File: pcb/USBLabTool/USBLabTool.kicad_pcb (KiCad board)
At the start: 4 copper layers, 79.4 x 56.2 mm, 236 parts, among them J1 Conn_01x06_Pin, J17 2x01, J19 T_N5V, J2 Conn_02x12_Odd_Even, J20 USB_C_Receptacle, K1 G5V-2, K2 G5V-2, Q1 STL11N3LLH6, SW1 TS02-66-73-BK-100-SCR-D, U1 AQY284SX, U10 MC33274ADR2G, U11 DG403, U12 STM32H562VGTx, U13 R1283K002A, U14 ST1L05APU33R, U15 ST1L05APU33R, U16 LTC1983ES6-5TRMPBF, U17 TCPP01-M12, U18 74HC245, U19 USBLC6-2SC6, U2 AQY284SX, U20 74HC245, U3 CD74HC4316, U4 LMP7718, U5 CD74HC4316, U6 LMP7718, U7 OPA863, U8 OPA863, U9 MC33274ADR2G, Y1 32.768kHz, Y2 NX2016SA-25M-EXS00A-CS08742

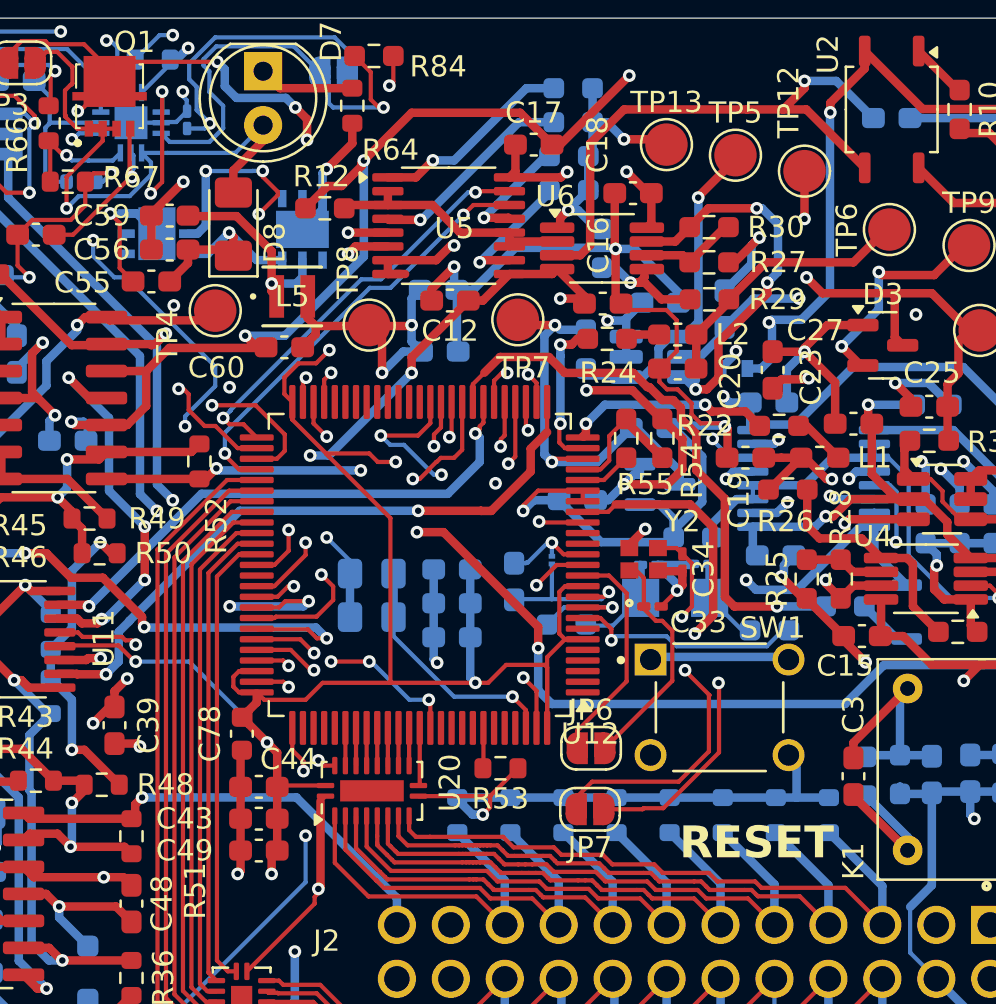
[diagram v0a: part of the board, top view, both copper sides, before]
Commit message: Update USBLabTool.kicad_pcb
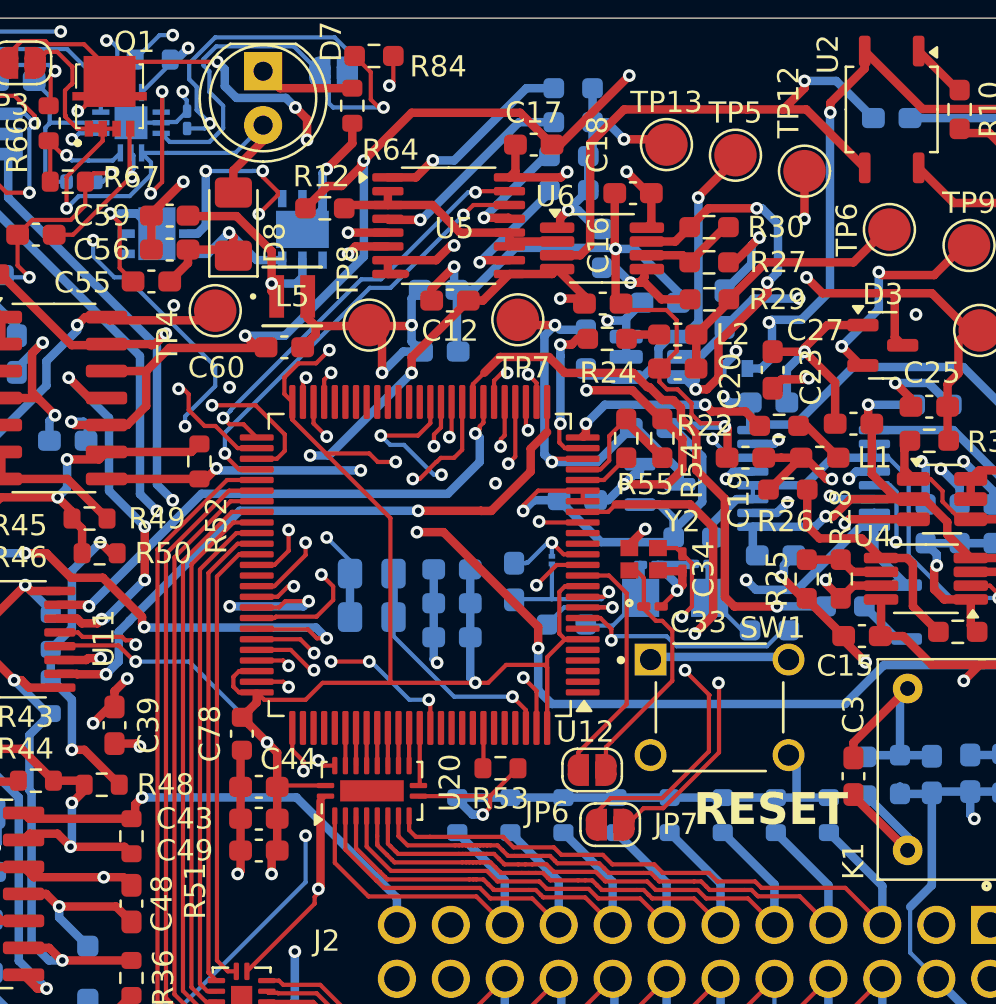
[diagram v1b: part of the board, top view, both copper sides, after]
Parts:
- moved JP7 1.20 mm to (151.8, 103.5)
- moved JP6 1.03 mm to (151.0, 101.0)
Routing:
- net RCC_OSC_IN: track 10.7 -> 11.7 mm
- net Net-(JP6-B): track 10.9 -> 11.9 mm
- net Net-(JP7-A): track 18.4 -> 17.7 mm
- net RCC_OSC_OUT: track 24.6 -> 24.0 mm
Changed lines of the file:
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@@
 		(tags "LQFP QFP")
 		(property "Reference" "U12"
-			(at -8.025 -7.95 0)
+			(at -7.794 -7.856 0)
 			(layer "F.SilkS")
 			(effects
@@
 	(footprint "Jumper:SolderJumper-2_P1.3mm_Open_RoundedPad1.0x1.5mm"
 		(layer "F.Cu")
-		(at 150.9 102.8 180)
+		(at 151.85 103.525 180)
 		(descr "SMD Solder Jumper, 1x1.5mm, rounded Pads, 0.3mm gap, open")
 		(tags "solder jumper open")
 		(property "Reference" "JP7"
-			(at 0 -1.8 0)
+			(at -3.1 0.025 0)
 			(layer "F.SilkS")
 			(effects
@@
 	(footprint "Jumper:SolderJumper-2_P1.3mm_Open_RoundedPad1.0x1.5mm"
 		(layer "F.Cu")
-		(at 150.95 99.925)
+		(at 151 100.95)
 		(descr "SMD Solder Jumper, 1x1.5mm, rounded Pads, 0.3mm gap, open")
 		(tags "solder jumper open")
 		(property "Reference" "JP6"
-			(at 0 -1.8 0)
+			(at -2.125 2 0)
 			(layer "F.SilkS")
 			(effects
@@
 	)
 	(gr_text "RESET"
-		(at 155.106 105.244 0)
+		(at 155.775 103.675 0)
 		(layer "F.SilkS")
 		(effects
@@
 	)
 	(segment
-		(start 150.3 99.1)
-		(end 150.3 99.925)
+		(start 152.625 92.625)
+		(end 152.625 97.85)
 		(width 0.2)
 		(layer "F.Cu")
@@
 	)
 	(segment
-		(start 152.625 96.775)
-		(end 150.3 99.1)
+		(start 150.35 100.125)
+		(end 150.35 100.95)
 		(width 0.2)
 		(layer "F.Cu")
@@
 	)
 	(segment
-		(start 152.625 92.625)
-		(end 152.625 96.775)
+		(start 152.625 97.85)
+		(end 150.35 100.125)
 		(width 0.2)
 		(layer "F.Cu")
@@
 	)
 	(segment
-		(start 156.5 97.45)
-		(end 156.5 100.075)
+		(start 149.331 91.294)
+		(end 148.375 92.25)
 		(width 0.2)
 		(layer "F.Cu")
@@
 	)
 	(segment
-		(start 149.331 91.294)
-		(end 148.375 92.25)
+		(start 156.5 97.45)
+		(end 156.525 97.425)
 		(width 0.2)
 		(layer "F.Cu")
@@
 	)
 	(segment
-		(start 151 101.5)
-		(end 150.25 102.25)
+		(start 151.2 103.525)
+		(end 151.2 102.95)
 		(width 0.2)
 		(layer "F.Cu")
@@
 	)
 	(segment
-		(start 156.525 97.425)
-		(end 156.5 97.45)
+		(start 151.875 102.275)
+		(end 154.3 102.275)
 		(width 0.2)
 		(layer "F.Cu")
@@
 	)
 	(segment
-		(start 150.25 102.25)
-		(end 150.25 102.8)
+		(start 151.2 102.95)
+		(end 151.875 102.275)
 		(width 0.2)
 		(layer "F.Cu")
@@
 	(segment
 		(start 156.5 100.075)
-		(end 155.075 101.5)
+		(end 156.5 97.45)
 		(width 0.2)
 		(layer "F.Cu")
@@
 	)
 	(segment
-		(start 155.375 96.275)
-		(end 156.525 97.425)
+		(start 154.3 102.275)
+		(end 156.5 100.075)
 		(width 0.2)
 		(layer "F.Cu")
@@
 	)
 	(segment
-		(start 155.075 101.5)
-		(end 151 101.5)
+		(start 156.525 97.425)
+		(end 155.375 96.275)
 		(width 0.2)
 		(layer "F.Cu")
@@
 	)
 	(segment
+		(start 129.215 70.79)
+		(end 129.215 72.915)
+		(width 0.2)
+		(layer "F.Cu")
+		(net 189)
+	)
+	(segment
 		(start 129.325 73.025)
 		(end 129.275 73.025)
@@
 	)
 	(segment
-		(start 129.275 73.025)
-		(end 126.556 75.744)
+		(start 129.215 72.915)
+		(end 129.325 73.025)
 		(width 0.2)
 		(layer "F.Cu")
@@
 	)
 	(segment
-		(start 129.215 70.79)
-		(end 129.215 72.735)
+		(start 129.275 73.025)
+		(end 126.556 75.744)
 		(width 0.2)
 		(layer "F.Cu")
@@
 	)
 	(segment
-		(start 153.435 91.91)
-		(end 153.435 93.25)
+		(start 151.925 99.6)
+		(end 154.775 96.75)
 		(width 0.2)
 		(layer "F.Cu")
@@
 	)
 	(segment
-		(start 151.6 99.925)
-		(end 154.775 96.75)
+		(start 153.435 91.91)
+		(end 153.435 93.25)
 		(width 0.2)
 		(layer "F.Cu")
@@
 	)
 	(segment
+		(start 151.65 100.95)
+		(end 151.65 99.875)
+		(width 0.2)
+		(layer "F.Cu")
+		(net 213)
+	)
+	(segment
 		(start 153.075 91.55)
 		(end 153.435 91.91)
@@
 	)
 	(segment
+		(start 151.65 99.875)
+		(end 151.925 99.6)
+		(width 0.2)
+		(layer "F.Cu")
+		(net 213)
+	)
+	(segment
 		(start 152.75 91.55)
 		(end 153.075 91.55)
@@
 	)
 	(segment
-		(start 153.375 102.8)
-		(end 151.55 102.8)
+		(start 154.35 102.75)
+		(end 153.425 102.75)
 		(width 0.2)
 		(layer "F.Cu")
@@
 	)
 	(segment
-		(start 156.975 100.125)
-		(end 154.35 102.75)
+		(start 152.65 103.525)
+		(end 152.5 103.525)
 		(width 0.2)
 		(layer "F.Cu")
@@
 	)
 	(segment
-		(start 154.35 102.75)
-		(end 153.425 102.75)
+		(start 154.975 90.5)
+		(end 155.25 90.775)
 		(width 0.2)
 		(layer "F.Cu")
@@
 	)
 	(segment
-		(start 156.95 96.85)
-		(end 156.975 96.875)
+		(start 156.975 100.125)
+		(end 154.35 102.75)
 		(width 0.2)
 		(layer "F.Cu")
@@
 	)
 	(segment
-		(start 156.975 96.875)
-		(end 156.975 100.125)
+		(start 154.1 90.5)
+		(end 154.975 90.5)
 		(width 0.2)
 		(layer "F.Cu")
@@
 	)
 	(segment
-		(start 154.975 90.5)
-		(end 155.25 90.775)
+		(start 156.975 96.875)
+		(end 156.975 100.125)
 		(width 0.2)
 		(layer "F.Cu")
@@
 	)
 	(segment
-		(start 154.1 90.5)
-		(end 154.975 90.5)
+		(start 153.425 102.75)
+		(end 152.65 103.525)
 		(width 0.2)
 		(layer "F.Cu")
@@
 	)
 	(segment
-		(start 153.425 102.75)
-		(end 153.375 102.8)
+		(start 156.95 96.85)
+		(end 156.875 96.925)
 		(width 0.2)
 		(layer "F.Cu")
@@
 	)
 	(segment
-		(start 156.95 96.85)
-		(end 156.875 96.925)
+		(start 155.7 91.225)
+		(end 155.7 93.25)
 		(width 0.2)
 		(layer "F.Cu")
@@
 	)
 	(segment
-		(start 155.7 91.225)
-		(end 155.7 93.25)
+		(start 156.95 96.85)
+		(end 156.975 96.875)
 		(width 0.2)
 		(layer "F.Cu")
